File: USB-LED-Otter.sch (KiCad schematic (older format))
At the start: 14 parts, among them J1 USB, J2 PAD, J3 LED, J4 PAD, J5 PAD, SW1 DFU, U1 MCP1700-3302E_SOT23, U2 STM32F072C8Ux

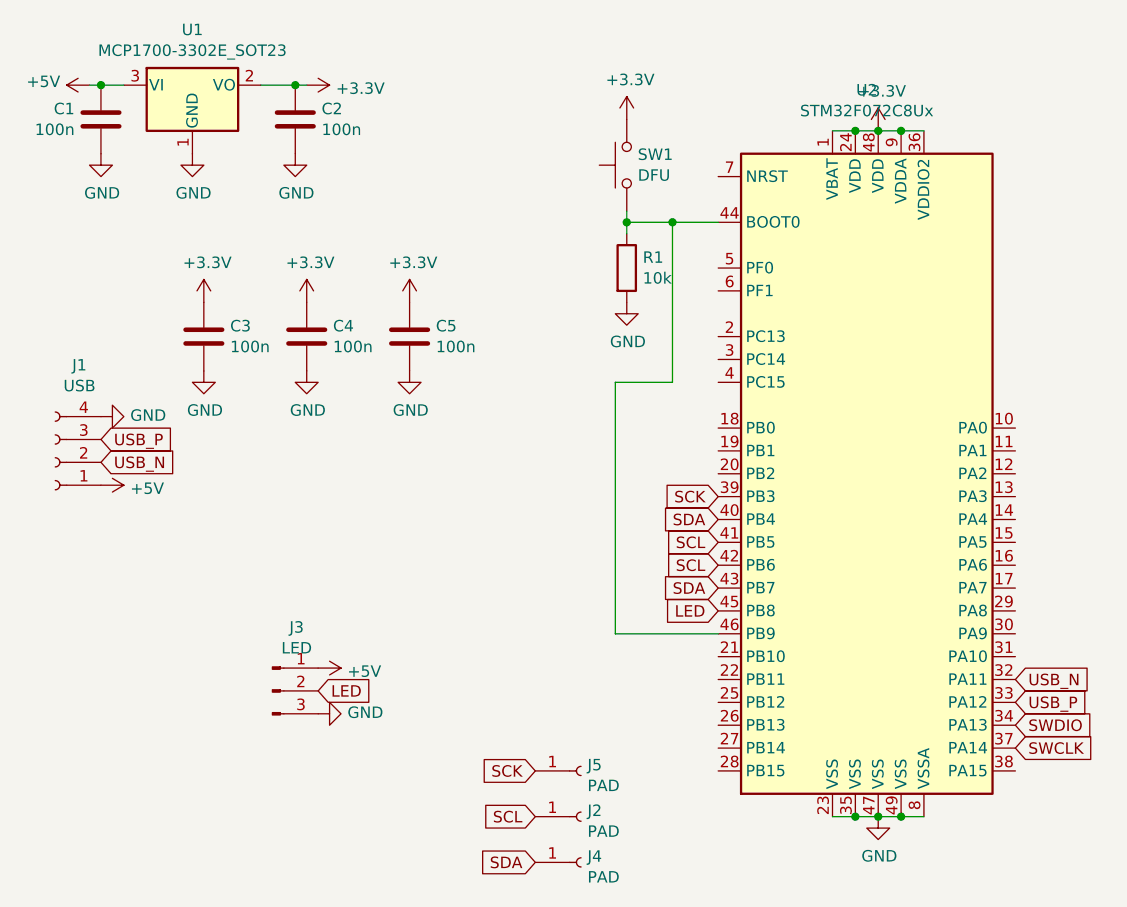
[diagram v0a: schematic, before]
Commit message: added example code
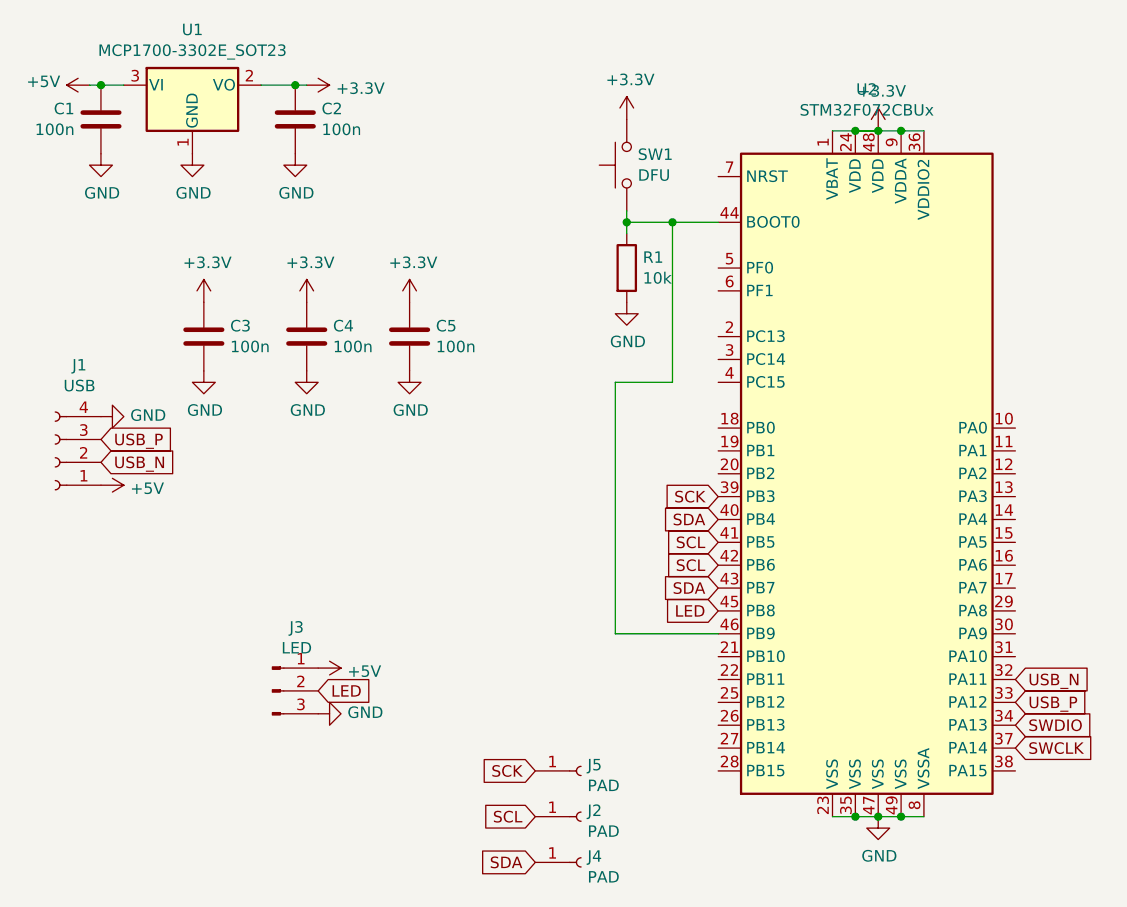
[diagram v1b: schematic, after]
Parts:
- removed U2: STM32F072C8Ux, otter:QFN-48-1EP_7x7mm_P0.5mm_EP2.6x2.6mm, symbol MCU_ST_STM32F0:STM32F072C8Ux
- added U2: STM32F072CBUx, otter:QFN-48-1EP_7x7mm_P0.5mm_EP2.6x2.6mm, symbol MCU_ST_STM32F0:STM32F072CBUx
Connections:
- net +3V3: now also U2.1 (VBAT), U2.24 (VDD), U2.36 (VDDIO2), U2.48 (VDD), U2.9 (VDDA)
- net GND: now also U2.23 (VSS), U2.35 (VSS), U2.47 (VSS), U2.49 (VSS), U2.8 (VSSA)
- net LED: now also U2.45 (PB8)
- net SCK: now also U2.39 (PB3)
- net SCL: now also U2.41 (PB5), U2.42 (PB6)
- net SDA: now also U2.40 (PB4), U2.43 (PB7)
- net SWCLK: now also U2.37 (PA14)
- net SWDIO: now also U2.34 (PA13)
- net USB_N: now also U2.32 (PA11)
- net USB_P: now also U2.33 (PA12)
- net at R1.1, SW1.1: now also U2.44 (BOOT0), U2.46 (PB9)
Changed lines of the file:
@@
 $EndDescr
-$Comp
-L MCU_ST_STM32F0:STM32F072C8Ux U2
-U 1 1 5DAD86AD
-P 5850 3150
-F 0 "U2" H 5800 4828 50  0000 C CNN
-F 1 "STM32F072C8Ux" H 5800 4737 50  0000 C CNN
-F 2 "otter:QFN-48-1EP_7x7mm_P0.5mm_EP2.6x2.6mm" H 5250 1750 50  0001 R CNN
-F 3 "http://www.st.com/st-web-ui/static/active/en/resource/technical/document/datasheet/DM00090510.pdf" H 5850 3150 50  0001 C CNN
-	1    5850 3150
-	1    0    0    -1
-$EndComp
 $Comp
 L Regulator_Linear:MCP1700-3302E_SOT23 U1
@@
 Text GLabel 2450 3100 2    50   Input ~ 0
 USB_N
-Wire Wire Line
-	6050 1650 5950 1650
-Connection ~ 5750 1650
-Wire Wire Line
-	5750 1650 5650 1650
 Connection ~ 5850 1650
-Wire Wire Line
-	5850 1650 5750 1650
-Connection ~ 5950 1650
-Wire Wire Line
-	5950 1650 5850 1650
-Wire Wire Line
-	6050 4650 5950 4650
-Connection ~ 5750 4650
-Wire Wire Line
-	5750 4650 5650 4650
 Connection ~ 5850 4650
-Wire Wire Line
-	5850 4650 5750 4650
-Connection ~ 5950 4650
-Wire Wire Line
-	5950 4650 5850 4650
 $Comp
 L power:GND #PWR0108
@@
 Text GLabel 6450 4350 2    50   Input ~ 0
 SWCLK
+$Comp
+L MCU_ST_STM32F0:STM32F072CBUx U2
+U 1 1 5DD36C6F
+P 5850 3150
+F 0 "U2" H 5800 4831 50  0000 C CNN
+F 1 "STM32F072CBUx" H 5800 4740 50  0000 C CNN
+F 2 "otter:QFN-48-1EP_7x7mm_P0.5mm_EP2.6x2.6mm" H 5250 1750 50  0001 R CNN
+F 3 "http://www.st.com/st-web-ui/static/active/en/resource/technical/document/datasheet/DM00090510.pdf" H 5850 3150 50  0001 C CNN
+	1    5850 3150
+	1    0    0    -1
+$EndComp
+Wire Wire Line
+	5750 1650 5850 1650
+Wire Wire Line
+	5750 4650 5850 4650
+Wire Wire Line
+	5650 4650 5750 4650
+Wire Wire Line
+	5850 4650 5950 4650
+Connection ~ 5750 4650
+Connection ~ 5950 4650
+Wire Wire Line
+	5950 4650 6050 4650
+Wire Wire Line
+	5650 1650 5750 1650
+Wire Wire Line
+	5850 1650 5950 1650
+Connection ~ 5750 1650
+Wire Wire Line
+	5750 1650 5850 1650
+Connection ~ 5950 1650
+Wire Wire Line
+	5950 1650 6050 1650
 $EndSCHEMATC
